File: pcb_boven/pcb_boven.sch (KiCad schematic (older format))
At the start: 30 parts, among them U1 miniIMU-9_v6, U2 openMV_M7_R2

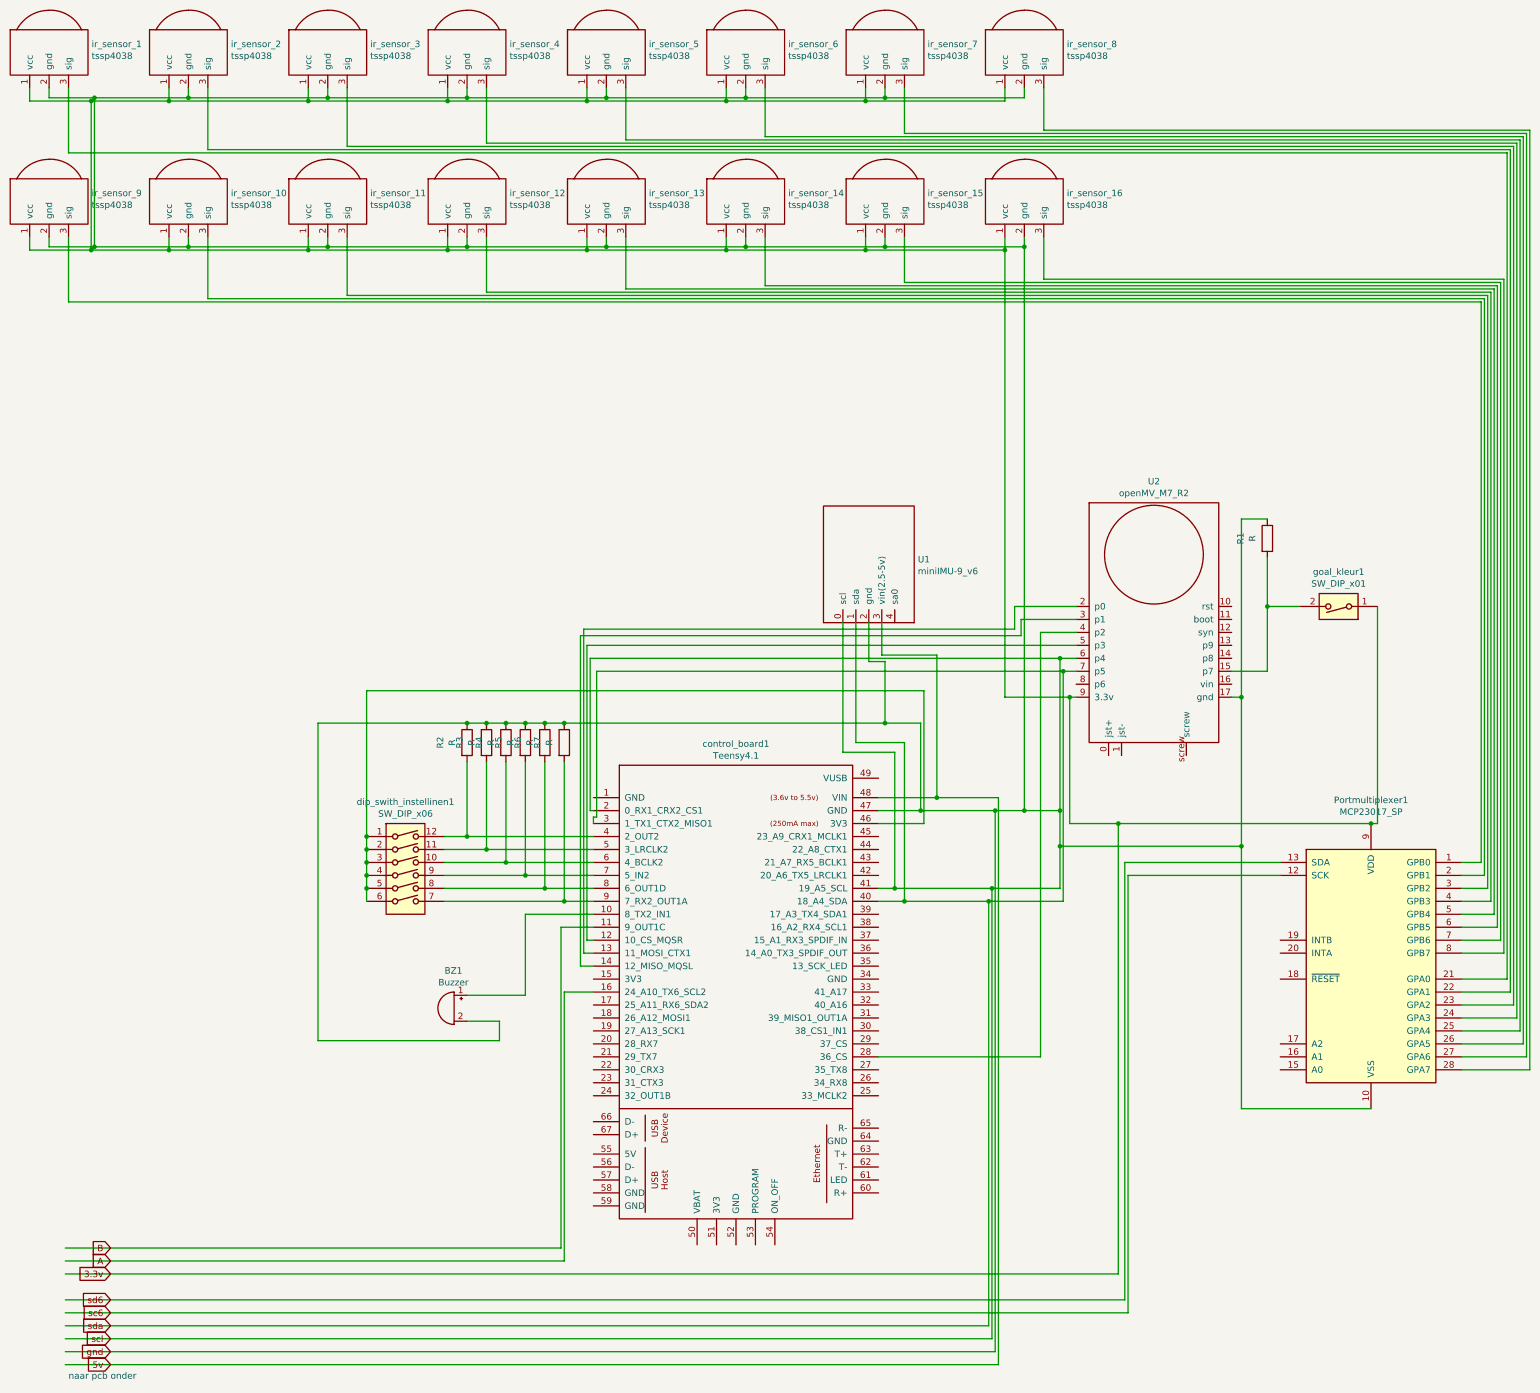
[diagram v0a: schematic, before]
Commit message: pcb
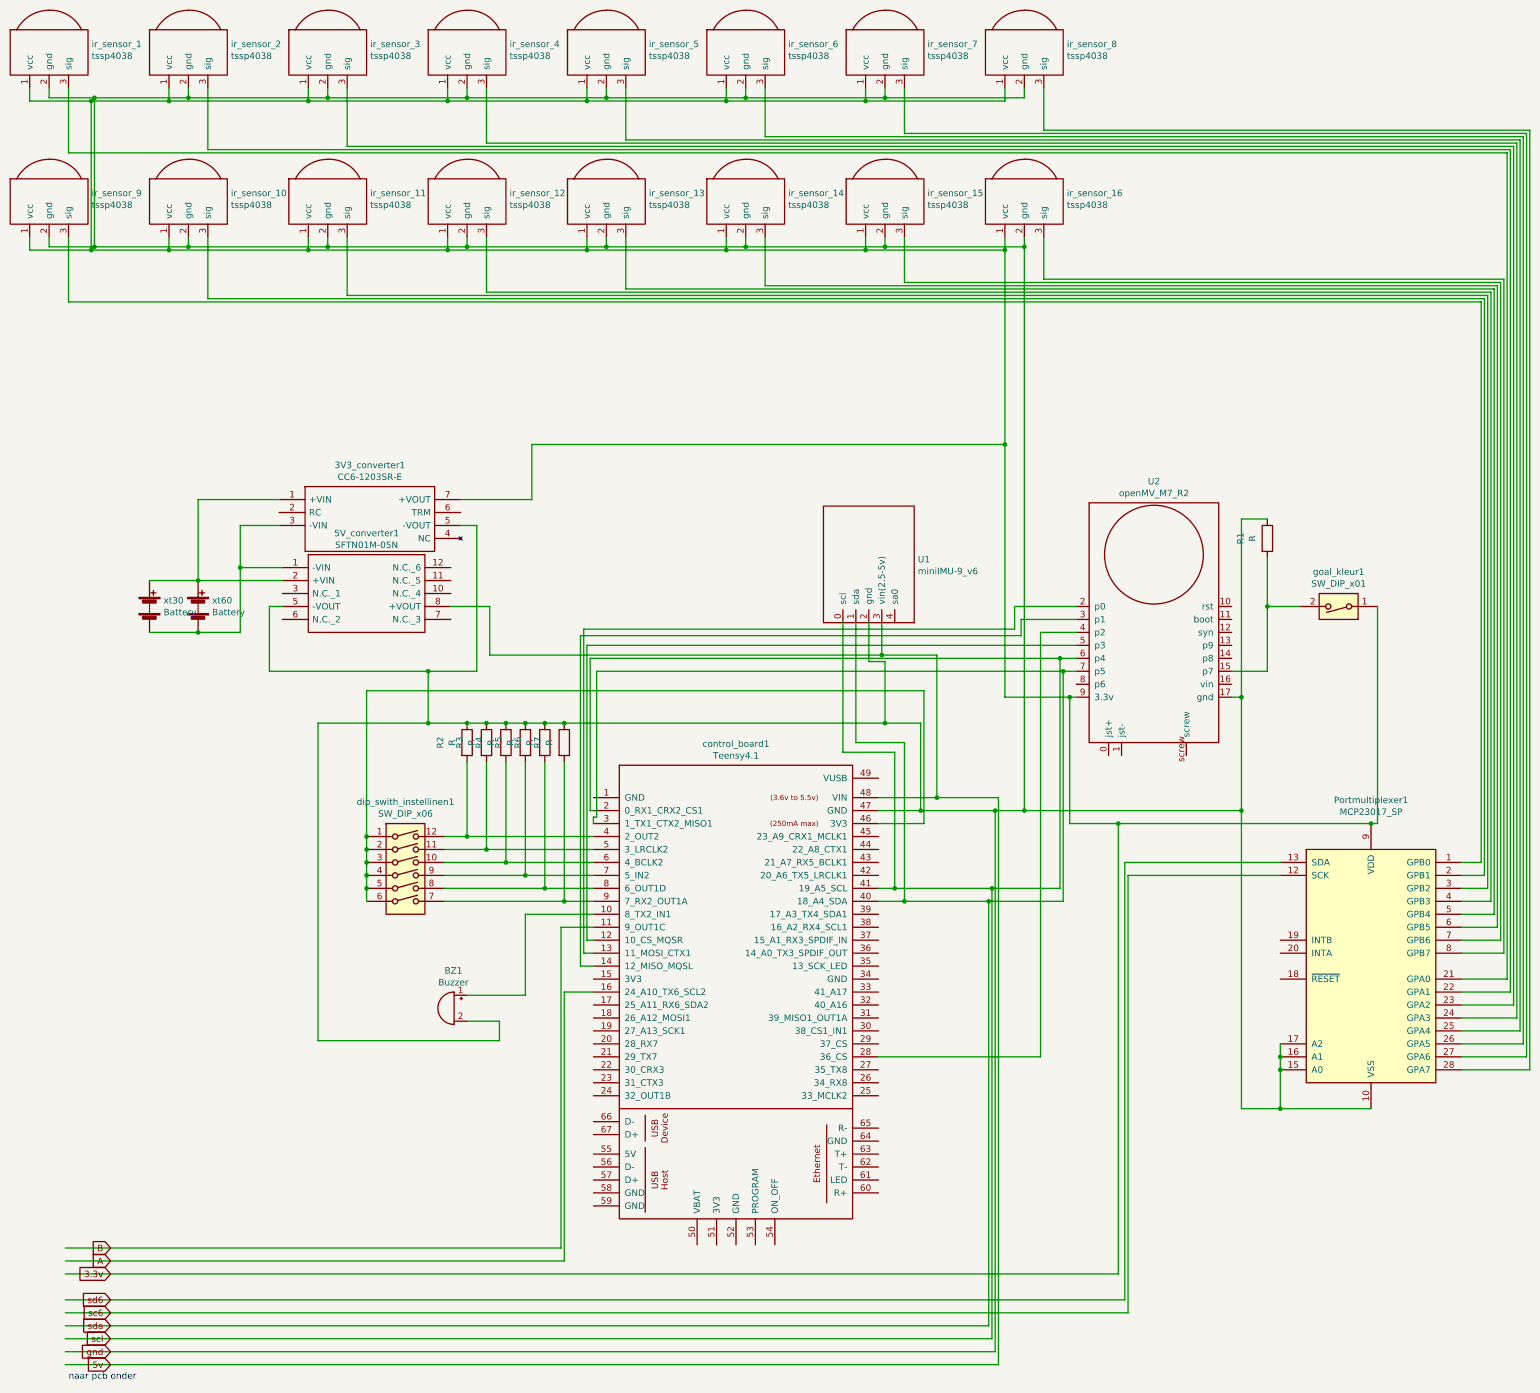
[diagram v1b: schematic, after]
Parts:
- added 3V3_converter1: CC6-1203SR-E, custom:CC60512SRE, symbol cc6-1203sr-e:CC6-1203SR-E
- added 5V_converter1: SFTN01M-05N, custom:SFTN01M05N, symbol sftn01m-05n:SFTN01M-05N
- added xt30: Battery, Connector_AMASS:AMASS_XT30U-F_1x02_P5.0mm_Vertical, symbol Device:Battery
- added xt60: Battery, Connector_AMASS:AMASS_XT60-F_1x02_P7.20mm_Vertical, symbol Device:Battery
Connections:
- wire segments 268 -> 294
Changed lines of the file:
@@
 	9950 5825 10025 5825
-Wire Wire Line
-	10025 5825 10025 6975
 Wire Wire Line
 	9075 10275 9075 6800
@@
 Wire Wire Line
 	8700 5825 8700 6800
-Wire Wire Line
-	11025 9000 10025 9000
-Wire Wire Line
-	10025 9000 10025 6975
-Connection ~ 10025 6975
 Wire Wire Line
 	825  2275 825  2350
@@
 Wire Wire Line
 	10025 4450 10025 5825
-Connection ~ 10025 5825
 $Comp
 L Device:Buzzer BZ1
@@
 	4500 7500 5025 7500
 Wire Wire Line
-	2900 6025 4050 6025
-Wire Wire Line
 	4050 8325 4300 8325
 Connection ~ 4050 6025
@@
 Wire Wire Line
 	8125 6700 8350 6700
-Wire Wire Line
-	8625 6975 10025 6975
 Connection ~ 8125 6700
 Wire Wire Line
 	8350 2350 8350 6700
 Connection ~ 8350 2350
-Connection ~ 8350 6700
-Wire Wire Line
-	8350 6700 8625 6700
-Wire Wire Line
-	8200 2375 8200 5825
+Wire Wire Line
+	8200 2375 8200 3875
 Wire Wire Line
 	8200 5825 8700 5825
@@
 Wire Wire Line
 	7350 7300 8100 7300
-Wire Wire Line
-	8625 5525 8625 6700
-Connection ~ 8625 6700
-Wire Wire Line
-	8625 6700 8625 6975
-Connection ~ 8625 6975
-Wire Wire Line
-	8625 6975 8625 7300
 Connection ~ 8100 7300
 Wire Wire Line
@@
 Wire Wire Line
 	8650 5625 8750 5625
+$Comp
+L Device:Battery xt60
+U 1 1 6666BA64
+P 1975 5125
+F 0 "xt60" H 2083 5171 50  0000 L CNN
+F 1 "Battery" H 2083 5080 50  0000 L CNN
+F 2 "Connector_AMASS:AMASS_XT60-F_1x02_P7.20mm_Vertical" V 1975 5185 50  0001 C CNN
+F 3 "https://eu.mouser.com/datasheet/2/813/xt60-2490175.pdf" V 1975 5185 50  0001 C CNN
+	1    1975 5125
+	1    0    0    -1
+$EndComp
+$Comp
+L Device:Battery xt30
+U 1 1 6666CC1A
+P 1600 5125
+F 0 "xt30" H 1708 5171 50  0000 L CNN
+F 1 "Battery" H 1708 5080 50  0000 L CNN
+F 2 "Connector_AMASS:AMASS_XT30U-F_1x02_P5.0mm_Vertical" V 1600 5185 50  0001 C CNN
+F 3 "https://eu.mouser.com/ProductDetail/DFRobot/FIT0586?qs=w%2Fv1CP2dgqouWR8IxqIK1w%3D%3D" V 1600 5185 50  0001 C CNN
+	1    1600 5125
+	1    0    0    -1
+$EndComp
+$Comp
+L cc6-1203sr-e:CC6-1203SR-E 3V3_converter1
+U 1 1 66680960
+P 2600 4300
+F 0 "3V3_converter1" H 3300 4565 50  0000 C CNN
+F 1 "CC6-1203SR-E" H 3300 4474 50  0000 C CNN
+F 2 "custom:CC60512SRE" H 3850 4400 50  0001 L CNN
+F 3 "https://product.tdk.com/system/files/dam/doc/product/power/switching-power/dc-dc-converter/catalog/cc-e_e.pdf" H 3850 4300 50  0001 L CNN
+F 4 "DC-DC Converters, On-board type, Output: 3.96W, 3.3V, Isolated type, Option: SMD type" H 3850 4200 50  0001 L CNN "Description"
+F 5 "8.8" H 3850 4100 50  0001 L CNN "Height"
+F 6 "TDK" H 3850 4000 50  0001 L CNN "Manufacturer_Name"
+F 7 "CC6-1203SR-E" H 3850 3900 50  0001 L CNN "Manufacturer_Part_Number"
+F 8 "967-CC6-1203SR-E" H 3850 3800 50  0001 L CNN "Mouser Part Number"
+F 9 "https://www.mouser.co.uk/ProductDetail/TDK-Lambda/CC6-1203SR-E?qs=Vwh6e7toGLi4J%2FzloL2n3g%3D%3D" H 3850 3700 50  0001 L CNN "Mouser Price/Stock"
+F 10 "CC6-1203SR-E" H 3850 3600 50  0001 L CNN "Arrow Part Number"
+F 11 "https://www.arrow.com/en/products/cc6-1203sr-e/tdk-lambda-americas?region=nac" H 3850 3500 50  0001 L CNN "Arrow Price/Stock"
+	1    2600 4300
+	1    0    0    -1
+$EndComp
+$Comp
+L sftn01m-05n:SFTN01M-05N 5V_converter1
+U 1 1 66681E5D
+P 2625 4825
+F 0 "5V_converter1" H 3275 5090 50  0000 C CNN
+F 1 "SFTN01M-05N" H 3275 4999 50  0000 C CNN
+F 2 "custom:SFTN01M05N" H 3775 4925 50  0001 L CNN
+F 3 "https://www.meanwell.com/webapp/product/search.aspx?prod=SFTN01-N" H 3775 4825 50  0001 L CNN
+F 4 "Isolated DC/DC Converters - SMD 1W 12Vin 5Vout 20-200mA SMT Unregulated" H 3775 4725 50  0001 L CNN "Description"
+F 5 "7.6" H 3775 4625 50  0001 L CNN "Height"
+F 6 "Mean Well" H 3775 4525 50  0001 L CNN "Manufacturer_Name"
+F 7 "SFTN01M-05N" H 3775 4425 50  0001 L CNN "Manufacturer_Part_Number"
+F 8 "709-SFTN01M-05N" H 3775 4325 50  0001 L CNN "Mouser Part Number"
+F 9 "https://www.mouser.co.uk/ProductDetail/MEAN-WELL/SFTN01M-05N?qs=A6eO%252BMLsxmQLvWwJN5Fn%252BQ%3D%3D" H 3775 4225 50  0001 L CNN "Mouser Price/Stock"
+	1    2625 4825
+	1    0    0    -1
+$EndComp
+Wire Wire Line
+	1600 4925 1975 4925
+Wire Wire Line
+	1975 5325 1600 5325
+Wire Wire Line
+	1975 5325 2300 5325
+Wire Wire Line
+	2300 5325 2300 4825
+Wire Wire Line
+	2300 4825 2625 4825
+Connection ~ 1975 5325
+Wire Wire Line
+	1975 4925 2625 4925
+Connection ~ 1975 4925
+Wire Wire Line
+	2300 4825 2300 4500
+Wire Wire Line
+	2300 4500 2600 4500
+Connection ~ 2300 4825
+Wire Wire Line
+	1975 4925 1975 4300
+Wire Wire Line
+	1975 4300 2600 4300
+Wire Wire Line
+	4000 4300 4550 4300
+Wire Wire Line
+	4550 4300 4550 3875
+Wire Wire Line
+	4550 3875 8200 3875
+Connection ~ 8200 3875
+Wire Wire Line
+	8200 3875 8200 5825
+Connection ~ 10025 5825
+Wire Wire Line
+	8625 5525 8625 7300
+Wire Wire Line
+	10025 5825 10025 6700
+Wire Wire Line
+	8350 6700 10025 6700
+Connection ~ 8350 6700
+Connection ~ 10025 6700
+Wire Wire Line
+	10025 6700 10025 9000
+Wire Wire Line
+	7250 5500 4225 5500
+Wire Wire Line
+	4225 5500 4225 5125
+Wire Wire Line
+	4225 5125 3925 5125
+Connection ~ 7250 5500
+Wire Wire Line
+	2625 5125 2525 5125
+Wire Wire Line
+	2525 5125 2525 5625
+Wire Wire Line
+	2525 5625 3750 5625
+Wire Wire Line
+	4125 5625 4125 4500
+Wire Wire Line
+	4125 4500 4000 4500
+Wire Wire Line
+	3750 5625 3750 6025
+Wire Wire Line
+	2900 6025 3750 6025
+Connection ~ 3750 5625
+Wire Wire Line
+	3750 5625 4125 5625
+Connection ~ 3750 6025
+Wire Wire Line
+	3750 6025 4050 6025
+Wire Wire Line
+	10325 8700 10325 8600
+Wire Wire Line
+	10325 8600 10325 8500
+Connection ~ 10325 8600
+Wire Wire Line
+	10325 8700 10325 9000
+Wire Wire Line
+	10025 9000 10325 9000
+Connection ~ 10325 8700
+Connection ~ 10325 9000
+Wire Wire Line
+	10325 9000 11025 9000
 $EndSCHEMATC
